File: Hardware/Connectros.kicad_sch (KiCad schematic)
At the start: 7 parts, among them J4 Sygnały, J5 Diagnostyka, J8 Zasilanie+CAN

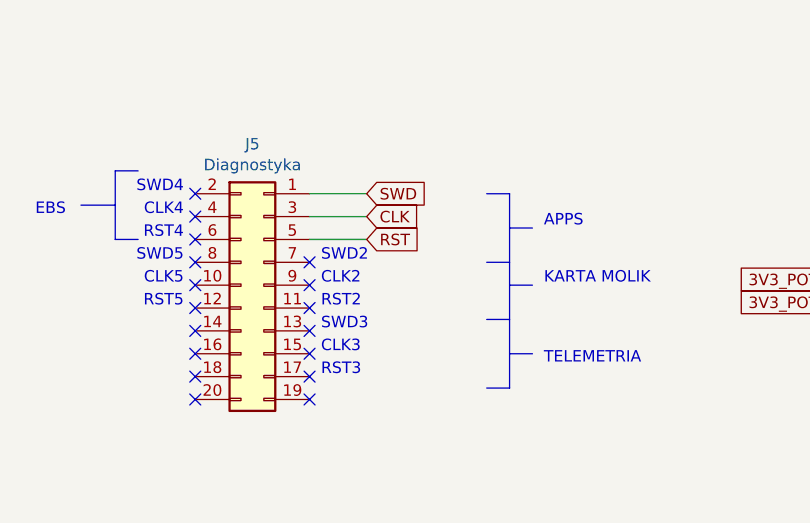
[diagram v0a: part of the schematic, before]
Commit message: Generated BOM
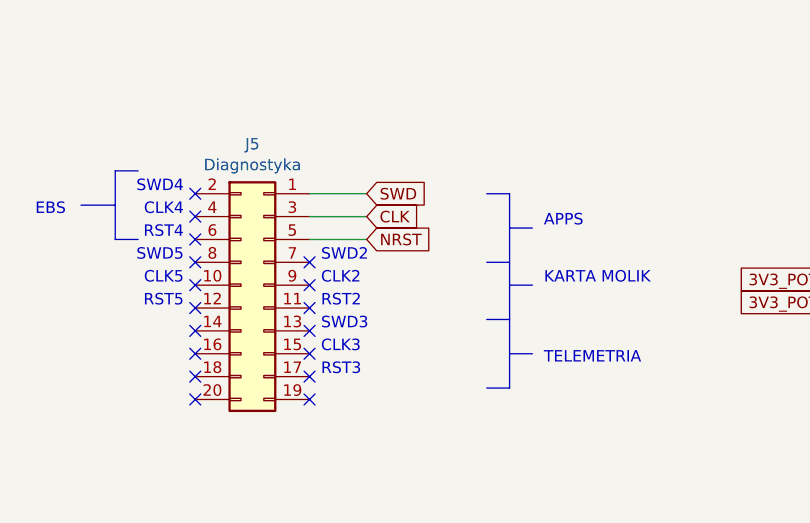
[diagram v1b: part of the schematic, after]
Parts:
- R11, R13, R15, R17: footprint Resistor_SMD:R_1206_3216Metric -> Resistor_SMD:R_0603_1608Metric_Pad0.98x0.95mm_HandSolder
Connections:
- net RST renamed NRST
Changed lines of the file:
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@@
     )
   )
-  (global_label "RST" (shape input) (at 133.35 85.725 0) (fields_autoplaced)
+  (global_label "NRST" (shape input) (at 133.35 85.725 0) (fields_autoplaced)
     (effects (font (size 1.27 1.27)) (justify left))
-    (property "Intersheet References" "${INTERSHEET_REFS}" (id 0) (at 139.1213 85.6456 0)
+    (property "Intersheet References" "${INTERSHEET_REFS}" (id 0) (at 140.4518 85.6456 0)
       (effects (font (size 1.27 1.27)) (justify left) hide)
     )
@@
     (property "Reference" "R17" (id 0) (at 260.985 95.25 90))
     (property "Value" "220R" (id 1) (at 260.985 97.155 90))
-    (property "Footprint" "Resistor_SMD:R_1206_3216Metric" (id 2) (at 262.255 90.932 90)
+    (property "Footprint" "Resistor_SMD:R_0603_1608Metric_Pad0.98x0.95mm_HandSolder" (id 2) (at 262.255 90.932 90)
       (effects (font (size 1.27 1.27)) hide)
     )
@@
     (property "Reference" "R11" (id 0) (at 196.85 88.265 90))
     (property "Value" "220R" (id 1) (at 195.58 86.36 90))
-    (property "Footprint" "Resistor_SMD:R_1206_3216Metric" (id 2) (at 195.58 91.948 90)
+    (property "Footprint" "Resistor_SMD:R_0603_1608Metric_Pad0.98x0.95mm_HandSolder" (id 2) (at 195.58 91.948 90)
       (effects (font (size 1.27 1.27)) hide)
     )
@@
     (property "Reference" "R15" (id 0) (at 260.985 88.265 90))
     (property "Value" "0R" (id 1) (at 260.985 86.36 90))
-    (property "Footprint" "Resistor_SMD:R_1206_3216Metric" (id 2) (at 262.255 88.392 90)
+    (property "Footprint" "Resistor_SMD:R_0603_1608Metric_Pad0.98x0.95mm_HandSolder" (id 2) (at 262.255 88.392 90)
       (effects (font (size 1.27 1.27)) hide)
     )
@@
     (property "Reference" "R13" (id 0) (at 196.85 95.25 90))
     (property "Value" "0R" (id 1) (at 195.58 97.155 90))
-    (property "Footprint" "Resistor_SMD:R_1206_3216Metric" (id 2) (at 195.58 94.488 90)
-      (effects (font (size 1.27 1.27)) hide)
-    )
+    (property "Footprint" "Resistor_SMD:R_0603_1608Metric_Pad0.98x0.95mm_HandSolder" (id 2) (at 195.58 94.488 90)
+      (effects (font (size 1.27 1.27)) hide)
+    )
